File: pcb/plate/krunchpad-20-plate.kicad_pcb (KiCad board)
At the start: 2 copper layers, 95.3 x 76.2 mm, 0 parts

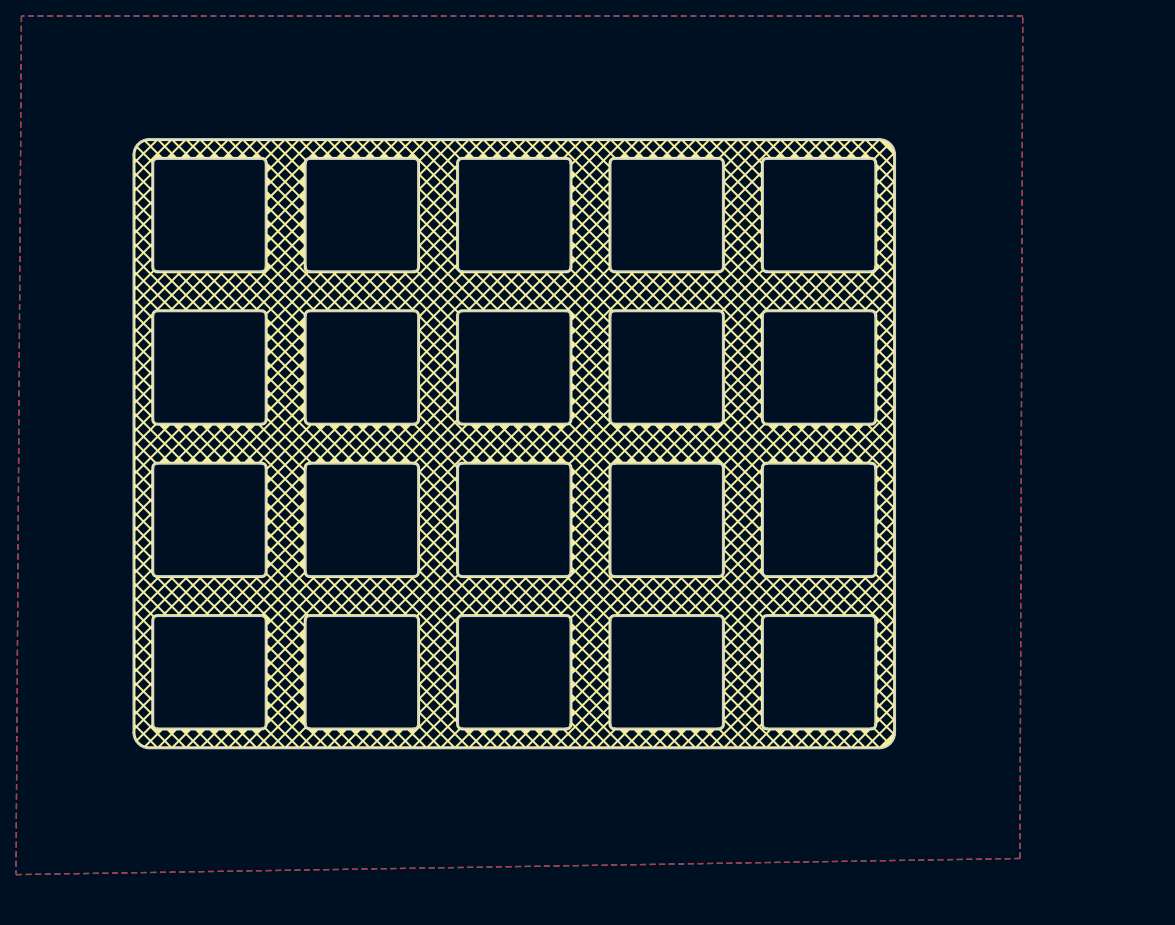
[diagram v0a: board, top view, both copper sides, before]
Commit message: updated plate
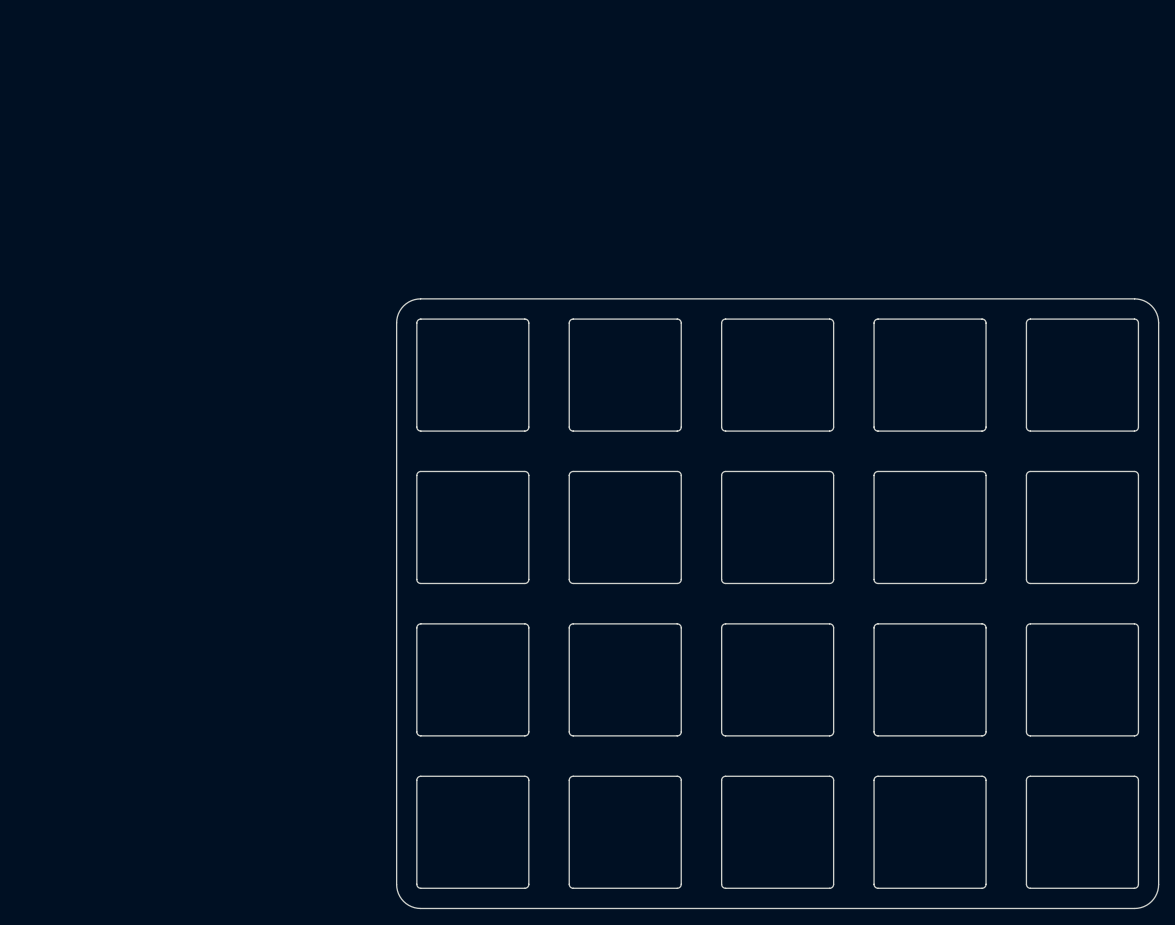
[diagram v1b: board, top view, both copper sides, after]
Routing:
- removed copper zone on B.Cu, net (none)
- removed copper zone on F.Cu, net (none)
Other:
- board size 95.3 x 76.2 mm -> 95.2 x 76.2 mm
